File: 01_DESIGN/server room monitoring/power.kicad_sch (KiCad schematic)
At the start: 17 parts, among them J1 Screw_Terminal_01x02, U1 LM2596S-5, U2 LM1117MP-3.3

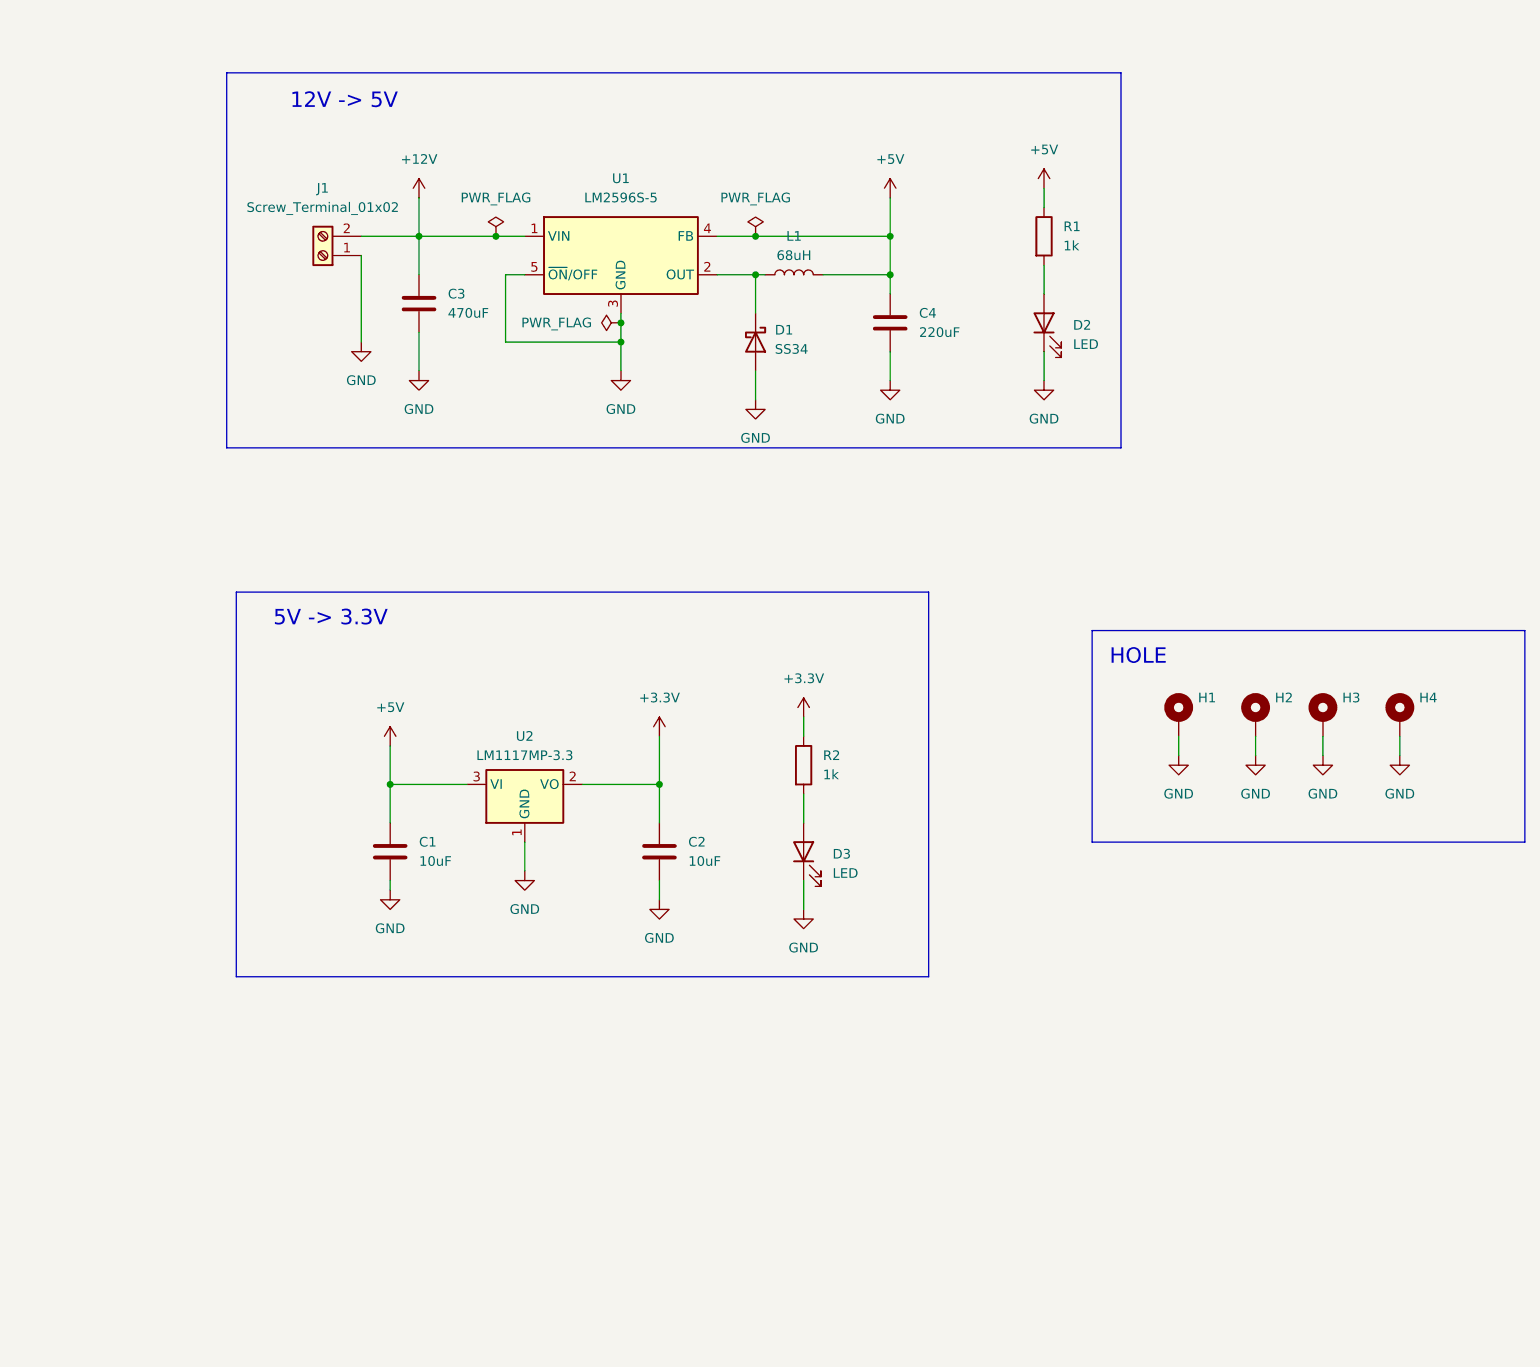
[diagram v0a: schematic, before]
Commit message: Update project files
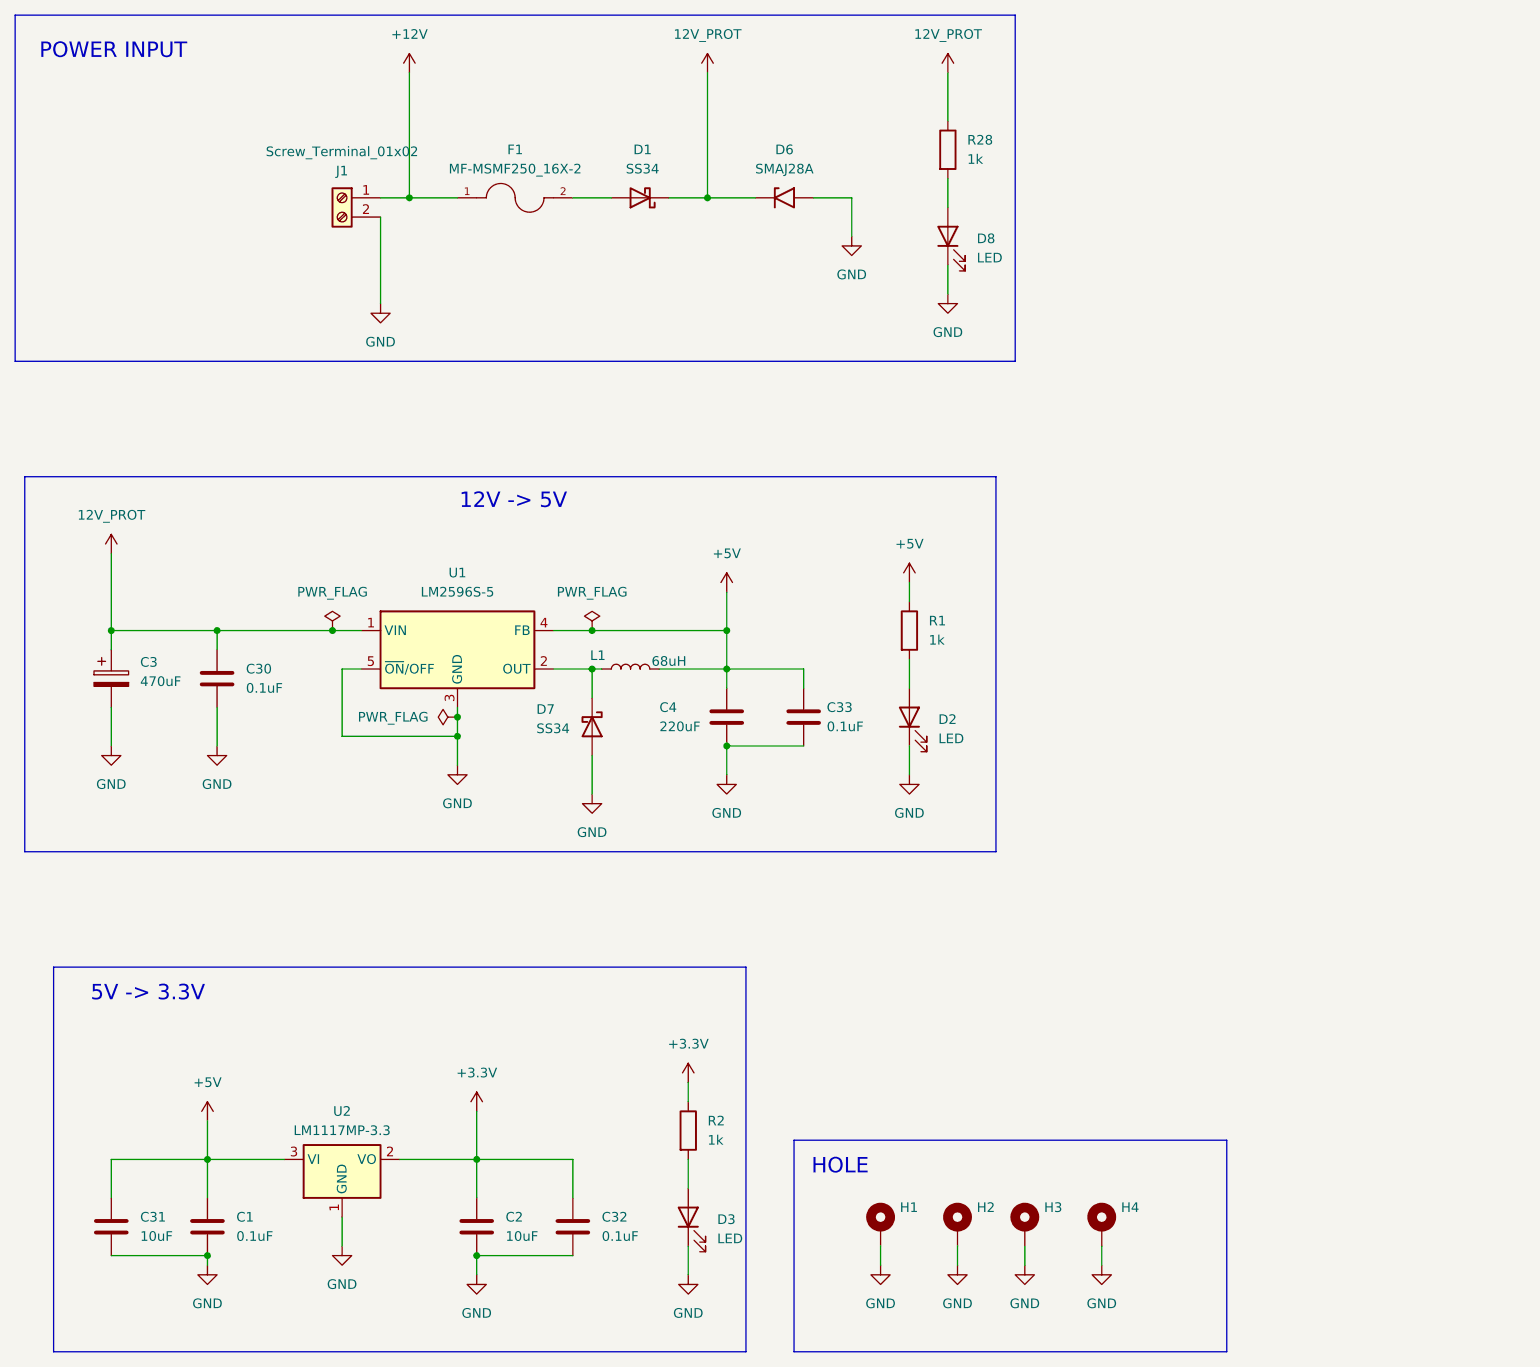
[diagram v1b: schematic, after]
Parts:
- removed C3: 470uF, symbol Device:C
- added C3: 470uF, Package_DIP:DIP-24_W7.62mm, symbol Device:C_Polarized
- added C30, C32, C33: 0.1uF, symbol Device:C
- added C31: 10uF, symbol Device:C
- added D6: SMAJ28A, Diode_SMD:D_SMA, symbol Diode:SMAJ28A
- added D7: SS34, Diode_SMD:D_SMA, symbol Diode:SS34
- added D8: LED, symbol Device:LED
- added F1: MF-MSMF250_16X-2, MF-MSMF250_16X-2:FUSER_MF-MSMF250_16X-2, symbol MF-MSMF250_16X-2:MF-MSMF250_16X-2
- added R28: 1k, symbol Device:R
- C1: value 10uF -> 0.1uF
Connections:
- net +12V: now also J1.1 (Pin_1), F1.1; no longer J1.2 (Pin_2), U1.1 (VIN)
- net +3.3V: now also C32.1
- net +5V: now also C31.1, C33.1
- net GND: now also J1.2 (Pin_2), C3.2, C30.2, C31.2, C32.2, C33.2, D6.2 (A2), D7.2 (A), D8.1 (K); no longer D1.2 (A), J1.1 (Pin_1)
- net at L1.2, U1.2 (OUT): now also D7.1 (K); no longer D1.1 (K)
- new net: D1.2 (A), F1.2
- new net: D8.2 (A), R28.2
- new net 12V_PROT: C3.1, C30.1, D1.1 (K), D6.1 (A1), R28.1, U1.1 (VIN)
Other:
- note added: "POWER INPUT"
- moved on the sheet: C1, C2, C4, D1, D2, D3, H1, H2, H3, H4, J1, L1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
